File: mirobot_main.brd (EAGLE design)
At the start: 100 x 40.6 mm, 25 parts, among them IC1 ULN2003AN, IC2 ULN2003AN, IC3 MEGA8-P, IC4 5V, IC5 3.3V, Q2 16M

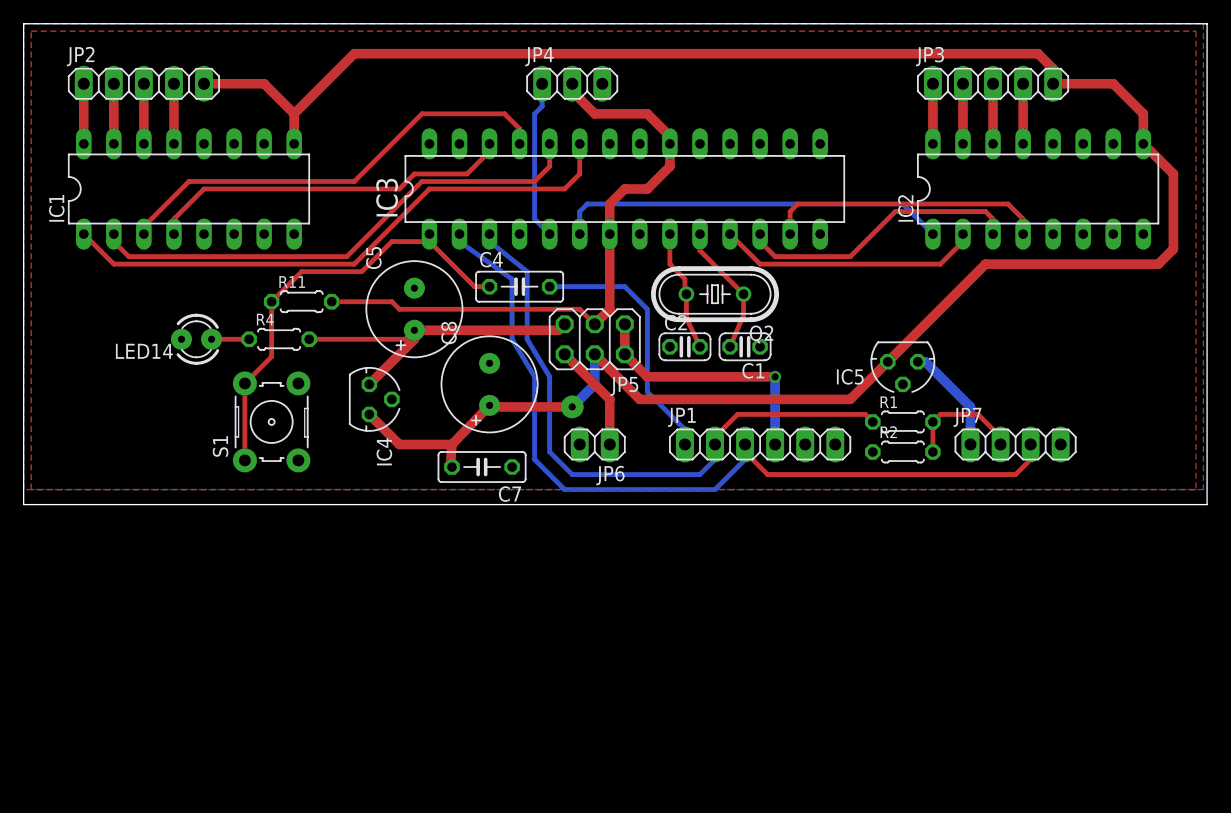
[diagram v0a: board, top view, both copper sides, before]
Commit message: Version 1.1 of the PCB
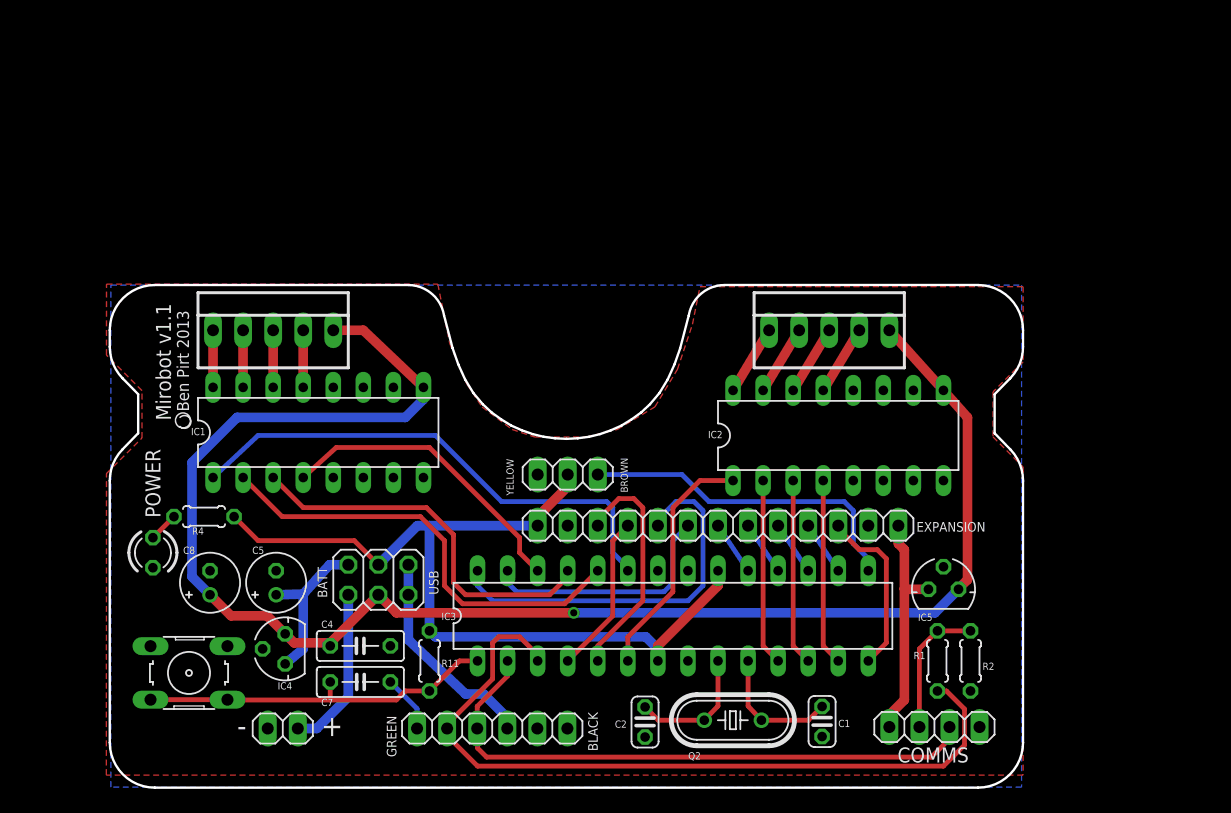
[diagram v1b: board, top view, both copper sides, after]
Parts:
- removed JP2: Stepper1, pinhead:1X05
- removed JP3: Stepper2, pinhead:1X05
- removed JP7: RF, pinhead:1X04
- removed LED14: POWER LED, led:LED3MM
- added COMMS: (no value), pinhead:1X04
- added EXPANSION: (no value), pinhead:1X13
- added POWER: (no value), led:LED3MM
- added X1, X2: 22-23-2051, con-molex:22-23-2051
- C5, C8: device rcl:E3,5-8 -> rcl:E2-5
- IC3: value MEGA8-P -> ATMEGA 328
- JP6: value Batt -> Battery
- moved IC3 36.3 mm to (54.9, 30.0)
- moved Q2 36.0 mm to (59.9, 21.1)
- moved C4 36.0 mm to (28.4, 24.4)
- moved JP6 35.7 mm to (21.9, 20.4)
- moved JP4 33.0 mm to (46.0, 41.9), turned to 180 degrees
- moved JP1 33.0 mm to (39.6, 20.4)
- moved C1 32.3 mm to (67.5, 21.0), turned to 90 degrees
- moved R11 32.2 mm to (34.3, 26.2), turned to 90 degrees
- moved C2 31.9 mm to (52.5, 21.0), turned to 90 degrees
- moved C8 29.0 mm to (15.7, 32.8)
- moved JP5 27.3 mm to (30.0, 33.0)
- moved IC2 26.8 mm to (68.8, 45.2)
- moved C5 25.9 mm to (21.3, 32.8)
- moved IC1 23.3 mm to (24.9, 45.5)
- moved S1 22.3 mm to (14.0, 25.1), turned to 180 degrees
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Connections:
- new net PB0: EXPANSION.3, IC3.14
- new net PB2: EXPANSION.4, IC3.16
- new net PB3: EXPANSION.5, IC3.17
- new net PB4: EXPANSION.6, IC3.18
- new net PB5: EXPANSION.7, IC3.19
- new net PC4: EXPANSION.8, IC3.27
- new net PC5: EXPANSION.9, IC3.28
- new net PD2: EXPANSION.10, IC3.4
- new net PD3: EXPANSION.11, IC3.5
- net +3V3: now also COMMS.1, EXPANSION.1; no longer JP7.1
- net +5V: now also EXPANSION.13, R4.2
- net GND: now also COMMS.4, EXPANSION.12, EXPANSION.2, POWER.K; no longer JP7.4, LED14.K
- net N$1: now also X1.1; no longer JP2.1
- net N$10: now also X2.3; no longer JP3.3
- net N$11: now also X2.4; no longer JP3.4
- net N$19: now also COMMS.2; no longer JP7.2
- net N$2: now also X1.2; no longer JP2.2
- net N$20: now also POWER.A; no longer LED14.A
- net N$3: now also X1.3; no longer JP2.3
- net N$4: now also X1.4; no longer JP2.4
- net N$8: now also X2.1; no longer JP3.1
- net N$9: now also X2.2; no longer JP3.2
- net RXD: now also COMMS.3; no longer JP7.3
- net SERVO: now also IC3.15; no longer IC3.5
- net V+: now also X1.5, X2.5; no longer JP2.5, JP3.5
- net VCC: no longer R4.2
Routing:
- net V+: track 183.0 -> 137.2 mm
- net PC5: track 0.00 -> 33.0 mm
- net PC4: track 0.00 -> 21.0 mm
- net +5V: track 53.1 -> 73.9 mm
- net RXD: track 70.4 -> 50.3 mm
- net PD3: track 0.00 -> 19.9 mm
- net EXT_RESET: track 21.8 -> 4.87 mm
- net SERVO: track 13.5 -> 28.5 mm
- net PB0: track 0.00 -> 14.6 mm
- net VCC: track 28.3 -> 13.8 mm
- net TXD: track 52.0 -> 66.1 mm
- net PD2: track 0.00 -> 13.5 mm
- net N$12: track 33.1 -> 20.6 mm
- net +3V3: track 9.20 -> 19.8 mm
- net N$17: track 24.0 -> 15.8 mm
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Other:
- board size 100 x 40.6 mm -> 77.2 x 42.5 mm
- board text added: "+"
- board text added: "-"
- board text added: "BATT"
- board text added: "BLACK"
- board text added: "BROWN"
- board text added: "Ben Pirt 2013"
- board text added: "GREEN"
- board text added: "Mirobot v1.1"
- board text added: "USB"
- board text added: "YELLOW"

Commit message: Version 1.2 of the Mirobot PCB
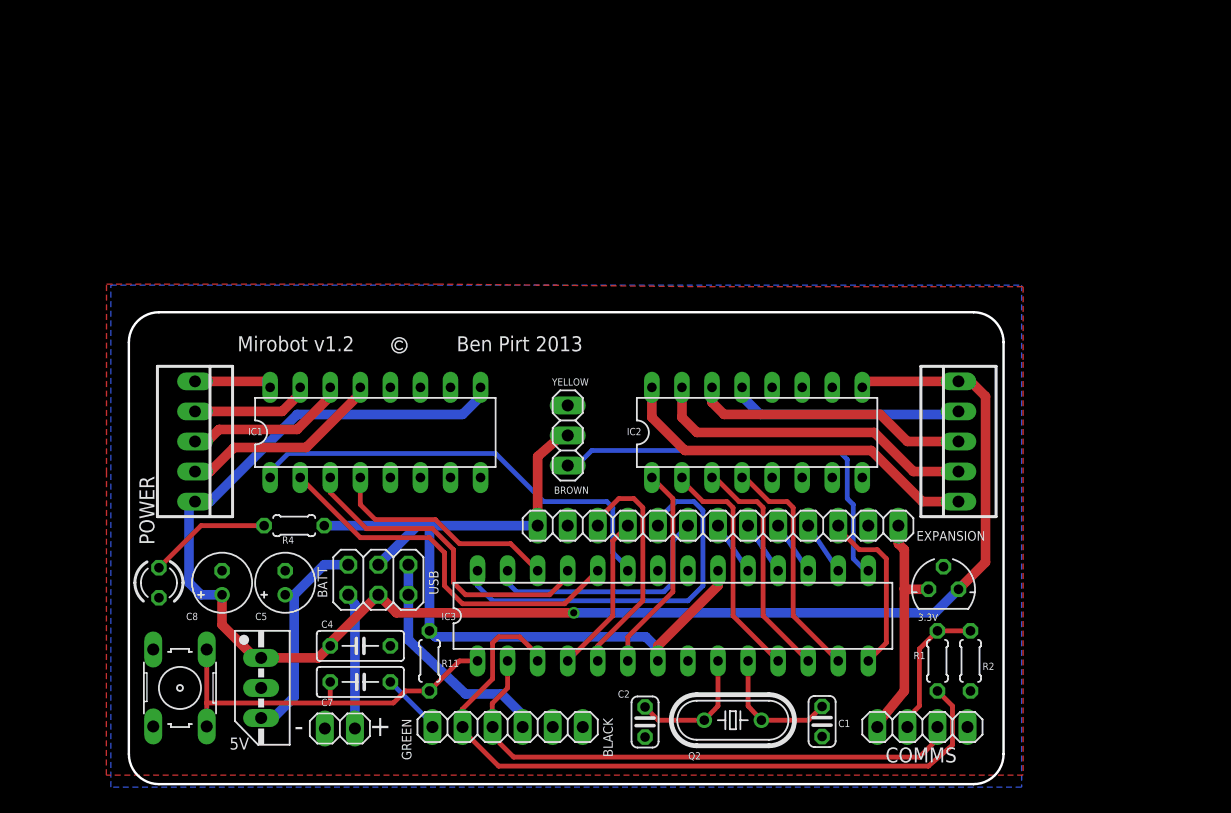
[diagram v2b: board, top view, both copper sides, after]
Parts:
- removed IC4: 5V, v-reg:78LXX
- added 5V: (no value), v-reg:78MXXS
- moved X2 14.4 mm to (79.0, 44.7), turned to 90 degrees
- moved X1 11.5 mm to (14.5, 44.7), turned to 270 degrees
- moved R4 7.66 mm to (22.9, 37.6)
- moved IC2 6.86 mm to (62.0, 45.5)
- moved IC1 4.83 mm to (29.7, 45.5)
- moved JP6 4.83 mm to (26.7, 20.4)
- moved JP4 3.30 mm to (46.0, 45.2), turned to 90 degrees
- moved POWER 2.59 mm to (11.4, 32.8)
- moved S1 1.48 mm to (13.2, 23.9), turned to 270 degrees
- moved JP1 1.30 mm to (40.9, 20.6)
- moved COMMS 1.02 mm to (75.9, 20.6)
- moved C8 1.02 mm to (16.8, 32.8)
- moved C5 0.76 mm to (22.1, 32.8)
- renumbered IC5 to 3.3V
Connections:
- net GND: now also 5V.GND; no longer IC4.GND
- net V+: now also 5V.IN; no longer IC4.IN
- net VCC: now also 5V.OUT; no longer IC4.OUT
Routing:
- net N$8: track 5.92 -> 31.4 mm
- net N$9: track 5.92 -> 27.8 mm
- net N$10: track 5.92 -> 23.5 mm
- net N$11: track 5.92 -> 19.8 mm
- net N$4: track 4.83 -> 17.2 mm
- net N$3: track 4.83 -> 13.8 mm
- net N$20: track 2.51 -> 10.4 mm
- net SERVO: track 28.5 -> 34.7 mm
- net N$5: track 25.9 -> 19.6 mm
- net N$13: track 43.6 -> 37.8 mm
- net N$14: track 37.8 -> 32.4 mm
- net N$2: track 4.83 -> 10.0 mm
- net N$15: track 32.5 -> 27.7 mm
- net VCC: track 13.8 -> 18.6 mm
- net N$16: track 15.8 -> 20.1 mm
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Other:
- board size 77.2 x 42.5 mm -> 73.9 x 39.9 mm
- board text added: "Mirobot v1.2"
- board text removed: "Mirobot v1.1"
